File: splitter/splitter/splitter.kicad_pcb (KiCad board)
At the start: 2 copper layers, 52 x 91.4 mm, 41 parts, among them J1 JACKIN, J2 JACKSEND, J3 JACKSEND2, J4 JACKRECV, J5 JACKRECV2, J6 JACKOUT, J7 Jack-DC, J8 Conn_01x08, J9 Conn_01x08, SW1 SW_BYPASS, SW2 SW_MODE, U1 TL074, U2 TLE2426xLP

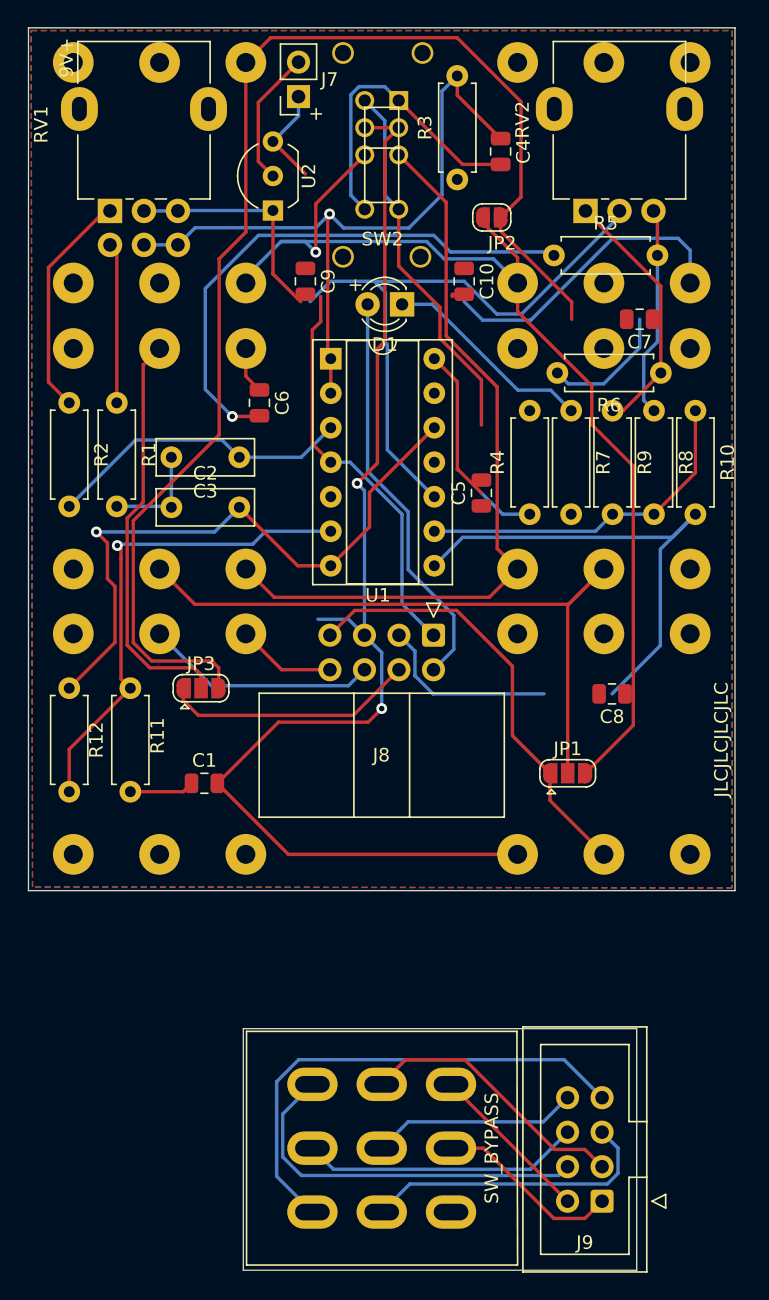
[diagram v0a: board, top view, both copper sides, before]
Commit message: redesign board: rev F
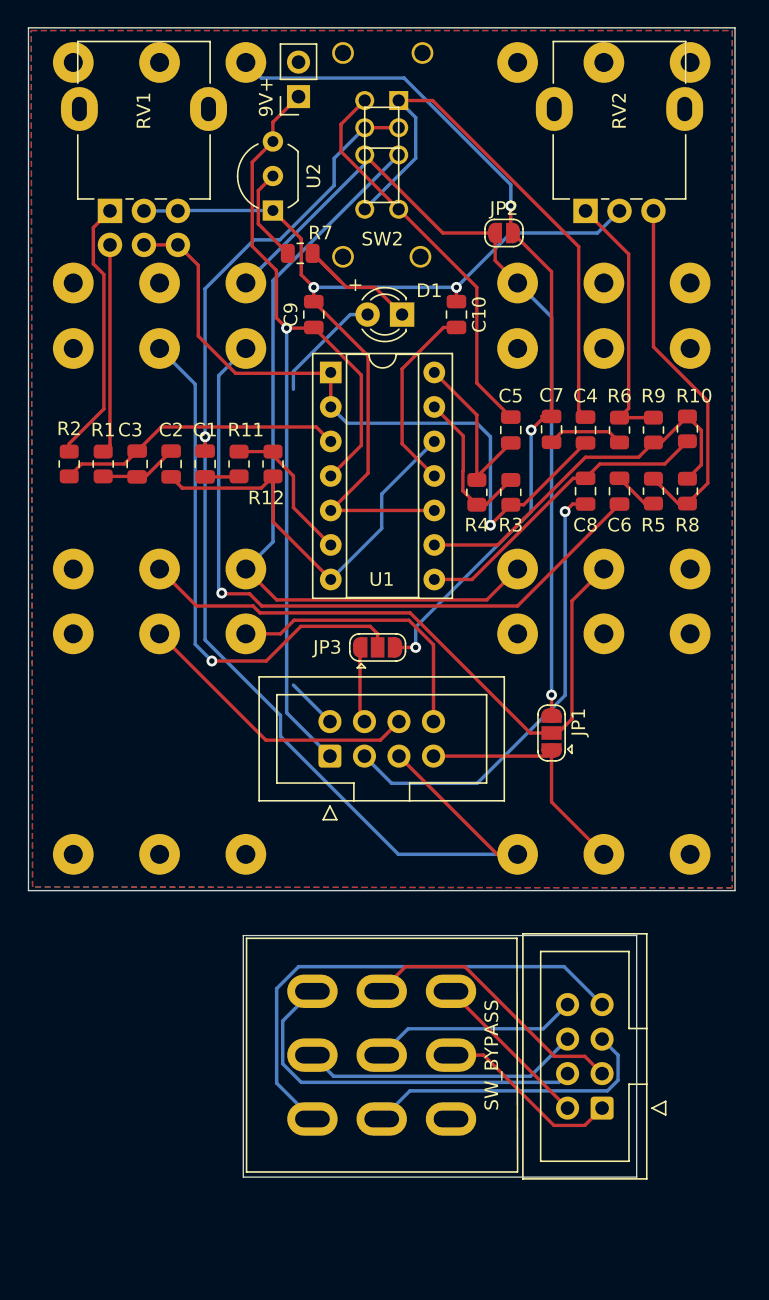
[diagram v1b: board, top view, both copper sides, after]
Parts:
- C2, C3: footprint Capacitor_THT:C_Rect_L7.0mm_W2.5mm_P5.00mm -> Capacitor_SMD:C_0805_2012Metric
- J7: footprint kicad-official/Connector_PinSocket_2.54mm.pretty:PinSocket_1x02_P2.54mm_Vertical -> Connector_PinSocket_2.54mm:PinSocket_1x02_P2.54mm_Vertical
- J8: footprint kicad-official/Connector_IDC.pretty:IDC-Header_2x04_P2.54mm_Horizontal -> Connector_IDC:IDC-Header_2x04_P2.54mm_Vertical
- J9: footprint kicad-official/Connector_IDC.pretty:IDC-Header_2x04_P2.54mm_Vertical -> Connector_IDC:IDC-Header_2x04_P2.54mm_Vertical
- JP1, JP3: footprint kicad-official/Jumper.pretty:SolderJumper-3_P1.3mm_Open_RoundedPad1.0x1.5mm -> Jumper:SolderJumper-3_P1.3mm_Open_RoundedPad1.0x1.5mm
- JP2: footprint kicad-official/Jumper.pretty:SolderJumper-2_P1.3mm_Open_RoundedPad1.0x1.5mm -> Jumper:SolderJumper-2_P1.3mm_Open_RoundedPad1.0x1.5mm
- R1, R10, R11, R12, R2, R3, R4, R5, R6, R8, R9: footprint Resistor_THT:R_Axial_DIN0207_L6.3mm_D2.5mm_P7.62mm_Horizontal -> Resistor_SMD:R_0805_2012Metric
- R7: value 10K -> 100K; footprint Resistor_THT:R_Axial_DIN0207_L6.3mm_D2.5mm_P7.62mm_Horizontal -> Resistor_SMD:R_0805_2012Metric
- U1: footprint kicad-official/Package_DIP.pretty:DIP-14_W7.62mm_Socket -> Package_DIP:DIP-14_W7.62mm_Socket
- U2: footprint kicad-official/Package_TO_SOT_THT.pretty:TO-92_Inline_Wide -> Package_TO_SOT_THT:TO-92_Inline_Wide
- moved C6 27.3 mm to (47.5, 43.5), turned to 90 degrees
- moved C1 23.5 mm to (17.0, 41.5), turned to 90 degrees
- moved R3 23.4 mm to (39.5, 43.6), turned to -90 degrees
- moved R7 23.1 mm to (24.0, 26.0), turned to 180 degrees
- moved R12 22.3 mm to (22.0, 41.5), turned to 90 degrees
- moved C4 21.4 mm to (45.0, 39.0), turned to 90 degrees
- moved R5 18.8 mm to (50.0, 43.5), turned to 90 degrees
- moved R11 18.3 mm to (19.5, 41.5)
- moved C8 15.0 mm to (45.0, 43.5), turned to -90 degrees
- moved JP3 13.3 mm to (29.7, 55.0)
- moved J8 11.7 mm to (26.2, 63.0), turned to 90 degrees
- moved C7 10.4 mm to (42.5, 39.0), turned to 90 degrees
- moved C3 7.53 mm to (12.0, 41.5), turned to -90 degrees
- moved SW1 6.85 mm to (30.0, 85.0)
- moved J9 6.85 mm to (46.2, 88.9)
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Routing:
- net /RECV_1: track 3.46 -> 51.7 mm, vias 0 -> 1
- net Net-(C6-Pad2): track 39.8 -> 3.27 mm, vias 1 -> 0
- net /RECV_2: track 96.4 -> 65.2 mm, vias 0 -> 3
- net +9V: track 37.2 -> 67.6 mm, vias 0 -> 1
- net Net-(U1B--): track 36.5 -> 10.8 mm, vias 1 -> 0
- net /OUT: track 13.5 -> 33.5 mm, vias 0 -> 1
- net /SEND_2: track 80.4 -> 62.3 mm
- net /HIGH: track 22.5 -> 40.5 mm
- net /LED: track 30.1 -> 12.3 mm
- net Net-(U1D-+): track 46.6 -> 30.9 mm, vias 1 -> 0
- net /INR: track 32.5 -> 18.1 mm
- net Net-(C8-Pad1): track 36.6 -> 22.8 mm
- net /RECVR: track 18.6 -> 5.13 mm
- net /OUTT: track 7.28 -> 20.6 mm
- net GNDD: track 33.6 -> 21.2 mm
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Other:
- board size 52 x 91.4 mm -> 52 x 84.6 mm
- board text added: "REV.F TONE SPLITTER 2025-04-03"
- board text removed: "JLCJLCJLCJLC"
- board text removed: "REV.E TONE SPLITTER 2023-09-28"
- board text removed: "switch shift up 6.85mm"
